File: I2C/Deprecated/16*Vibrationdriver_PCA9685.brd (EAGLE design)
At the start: 58.9 x 22.1 mm, 32 parts, among them IC1 LM317MDTRKG, U1 PCA9685, U2 ULN2803ADWR, U3 ULN2803ADWR

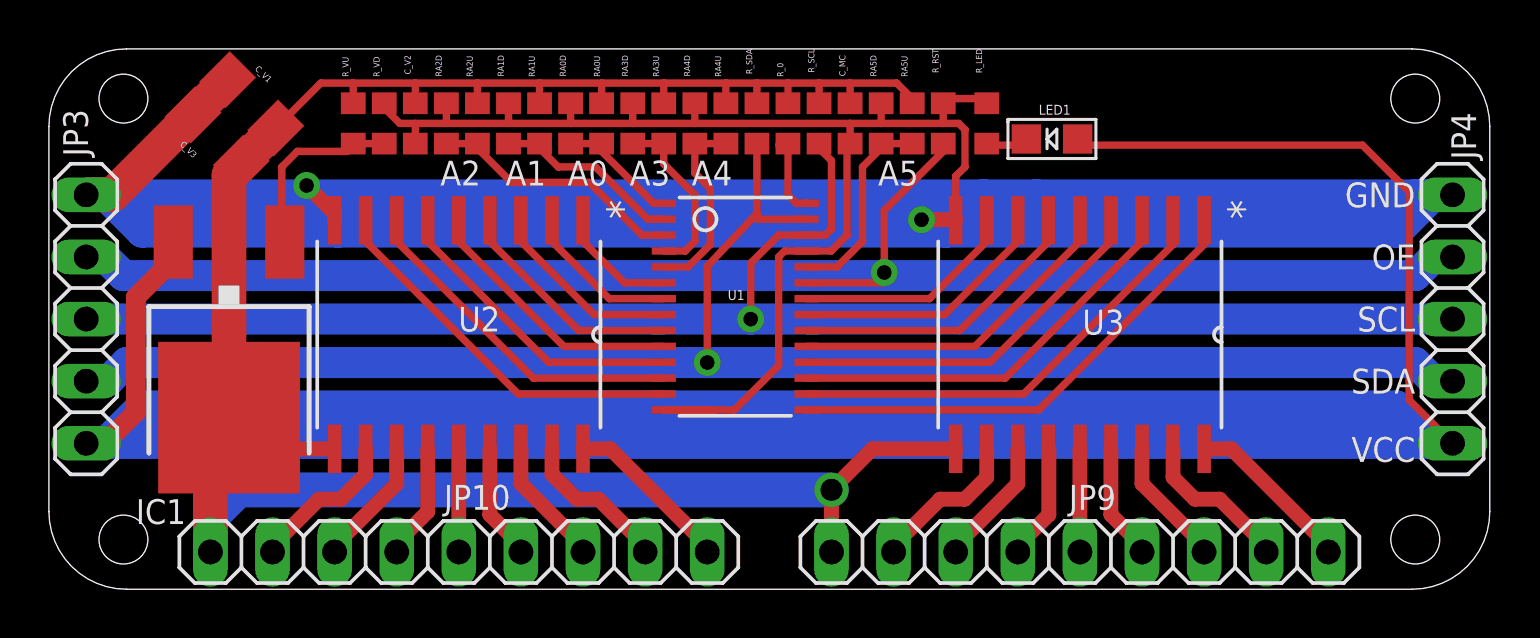
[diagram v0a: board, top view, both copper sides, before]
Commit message: Updates
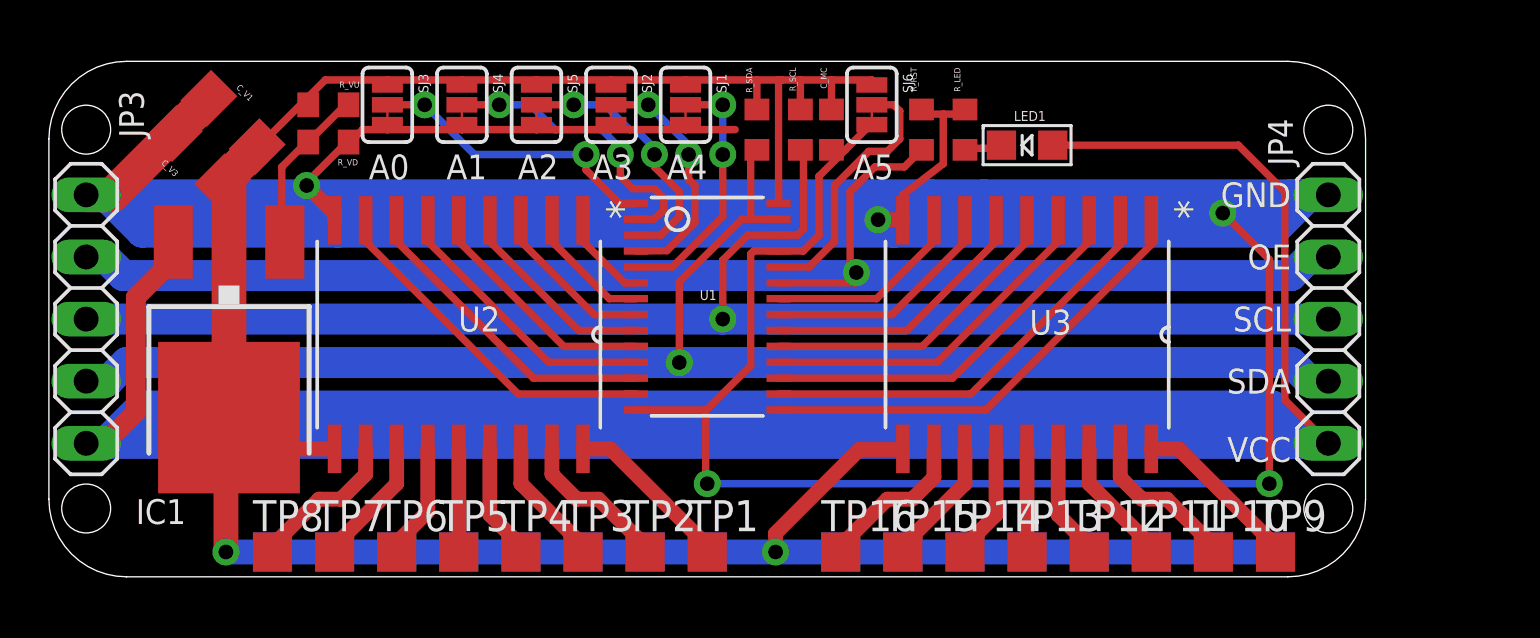
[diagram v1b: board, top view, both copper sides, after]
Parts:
- removed C_V2: 100n, thar:603
- removed JP10, JP9: (no value), pinhead:1X09
- removed RA0D, RA1D, RA2D, RA3D, RA4D, RA5D: 10k, thar:603
- removed RA0U, RA1U, RA2U, RA3U, RA4U, RA5U, R_0: 0, thar:603
- added SJ1, SJ2, SJ3, SJ4, SJ5, SJ6: (no value), SparkFun-Retired:SJ_3_PASTE2&3
- added TP1, TP10, TP11, TP12, TP13, TP14, TP15, TP16, TP17, TP18, TP19, TP2, TP20, TP21, TP22, TP23, TP24, TP25, TP26, TP27, TP28, TP29, TP3, TP30, TP31, TP32, TP4, TP5, TP6, TP7, TP8, TP9: TPTP16SQ, testpad:TP16SQ
- moved JP4 5.08 mm to (58.5, 15.1)
- moved R_VD 2.41 mm to (17.7, 22.4), turned to 180 degrees
- moved U3 2.16 mm to (46.2, 14.5)
- moved R_VU 1.27 mm to (17.7, 23.9), turned to 0 degrees
- moved U1 1.14 mm to (33.1, 15.6)
- moved C_V1 1.08 mm to (13.8, 23.2)
- moved C_V3 1.08 mm to (12.3, 21.7)
- moved LED1 1.05 mm to (46.2, 22.2)
- moved R_RST 0.92 mm to (41.9, 22.9)
- moved R_LED 0.92 mm to (43.7, 22.9)
- moved C_MC 0.80 mm to (38.2, 22.9)
- moved R_SCL 0.80 mm to (37.0, 22.9)
- moved R_SDA 0.25 mm to (35.2, 22.9)
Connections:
- removed net A0: RA0D.1, RA0U.2, U1.1
- removed net A1: RA1D.1, RA1U.2, U1.2
- removed net A2: RA2D.1, RA2U.2, U1.3
- removed net A3: RA3D.1, RA3U.2, U1.4
- removed net A4: RA4D.1, RA4U.2, U1.5
- removed net A5: RA5D.1, RA5U.2, U1.24
- removed net N$2: R_0.2, U1.28
- net +3V3: now also SJ1.1, SJ2.1, SJ3.1, SJ4.1, SJ5.1, SJ6.1, TP17.TP, TP18.TP, TP19.TP, TP20.TP, TP21.TP, TP22.TP, TP23.TP, TP24.TP, TP25.TP, TP26.TP, TP27.TP, TP28.TP, TP29.TP, TP30.TP, TP31.TP, TP32.TP, U1.28; no longer C_V2.2, JP10.9, JP9.9, RA0U.1, RA1U.1, RA2U.1, RA3U.1, RA4U.1, RA5U.1, R_0.1
- net GND: now also SJ1.2, SJ1.3, SJ2.2, SJ2.3, SJ3.2, SJ3.3, SJ4.2, SJ4.3, SJ5.2, SJ5.3, SJ6.2, SJ6.3, U1.1, U1.2, U1.24, U1.3, U1.4, U1.5; no longer C_V2.1, RA0D.2, RA1D.2, RA2D.2, RA3D.2, RA4D.2, RA5D.2
- net N$14: now also TP1.TP; no longer JP10.1
- net N$19: now also TP2.TP; no longer JP10.2
- net N$20: now also TP3.TP; no longer JP10.3
- net N$21: now also TP4.TP; no longer JP10.4
- net N$22: now also TP5.TP; no longer JP10.5
- net N$23: now also TP6.TP; no longer JP10.6
- net N$24: now also TP7.TP; no longer JP10.7
- net N$25: now also TP8.TP; no longer JP10.8
- net N$26: now also TP9.TP; no longer JP9.1
- net N$27: now also TP10.TP; no longer JP9.2
- net N$28: now also TP11.TP; no longer JP9.3
- net N$29: now also TP12.TP; no longer JP9.4
- net N$30: now also TP13.TP; no longer JP9.5
- net N$31: now also TP14.TP; no longer JP9.6
- net N$32: now also TP15.TP; no longer JP9.7
- net N$33: now also TP16.TP; no longer JP9.8
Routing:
- net GND: track 243.5 -> 325.8 mm, vias 2 -> 15
- net OE: track 88.5 -> 64.0 mm
- net +3V3: track 99.2 -> 119.2 mm, vias 1 -> 2
- net VCC: track 202.9 -> 183.4 mm
- net A2: track 10.6 -> 0.00 mm
- net A5: track 8.31 -> 0.00 mm
- net A4: track 7.94 -> 0.00 mm
- net A1: track 7.75 -> 0.00 mm
- net A3: track 7.48 -> 0.00 mm
- net SCL: track 66.3 -> 60.4 mm
- net SDA: track 68.5 -> 62.9 mm
- net A0: track 5.29 -> 0.00 mm
- net N$2: track 4.02 -> 0.00 mm
- net N$18: track 9.30 -> 7.82 mm
- net PWM7: track 15.6 -> 14.5 mm
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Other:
- board size 58.9 x 22.1 mm -> 53.8 x 21.1 mm
